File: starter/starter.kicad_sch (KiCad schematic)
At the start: 44 parts, among them J1 Conn_01x04_MountingPin, J2 Conn_01x02, J3 Conn_01x04_MountingPin, J4 Conn_01x04_MountingPin, J5 Conn_01x02_MountingPin, Q1 Q_NMOS_GDS, SW1 SW_Coded_SH-7050, SW2 SW_Coded_SH-7050, U1 MCP100-475D, U2 LM1117DT-ADJ, U3 PCF8574RGTR, U4 74HC688, U5 MCP14A1201xMNY

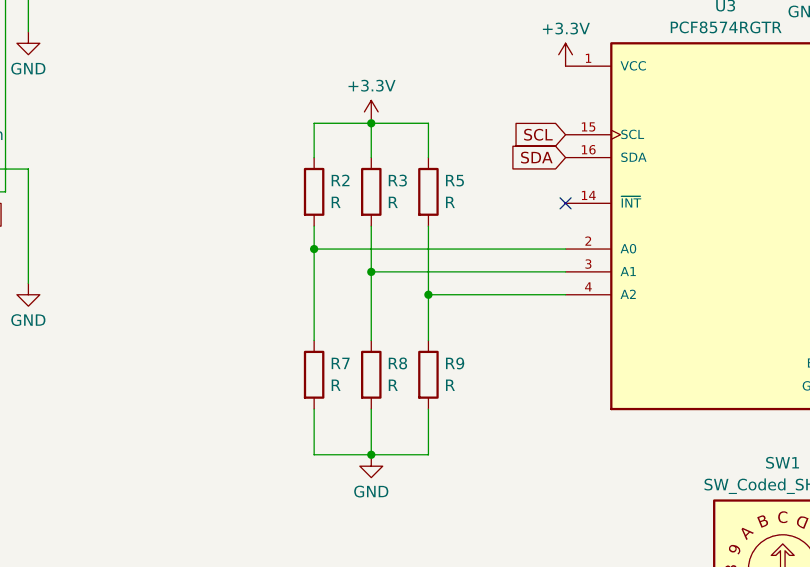
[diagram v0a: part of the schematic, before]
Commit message: updates
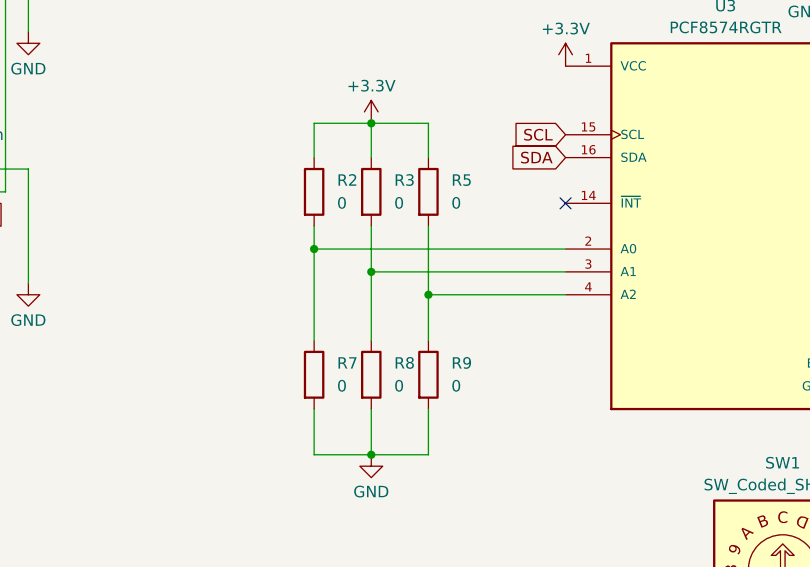
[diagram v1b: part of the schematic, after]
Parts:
- R2, R3, R5, R7, R8, R9: value R -> 0
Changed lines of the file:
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@@
 		(fields_autoplaced yes)
 		(property "Reference" "R5"
-			(at 94.488 138.4878 0)
+			(at 95.25 138.4299 0)
 			(effects
 				(font
@@
 			)
 		)
-		(property "Value" "R"
-			(at 94.488 140.9121 0)
+		(property "Value" "0"
+			(at 95.25 140.9699 0)
 			(effects
 				(font
@@
 		(fields_autoplaced yes)
 		(property "Reference" "R3"
-			(at 88.138 138.4878 0)
+			(at 88.9 138.4299 0)
 			(effects
 				(font
@@
 			)
 		)
-		(property "Value" "R"
-			(at 88.138 140.9121 0)
+		(property "Value" "0"
+			(at 88.9 140.9699 0)
 			(effects
 				(font
@@
 		(fields_autoplaced yes)
 		(property "Reference" "R9"
-			(at 94.488 158.8078 0)
+			(at 95.25 158.7499 0)
 			(effects
 				(font
@@
 			)
 		)
-		(property "Value" "R"
-			(at 94.488 161.2321 0)
+		(property "Value" "0"
+			(at 95.25 161.2899 0)
 			(effects
 				(font
@@
 		(fields_autoplaced yes)
 		(property "Reference" "R8"
-			(at 88.138 158.8078 0)
+			(at 88.9 158.7499 0)
 			(effects
 				(font
@@
 			)
 		)
-		(property "Value" "R"
-			(at 88.138 161.2321 0)
+		(property "Value" "0"
+			(at 88.9 161.2899 0)
 			(effects
 				(font
@@
 		(fields_autoplaced yes)
 		(property "Reference" "R2"
-			(at 81.788 138.4878 0)
+			(at 82.55 138.4299 0)
 			(effects
 				(font
@@
 			)
 		)
-		(property "Value" "R"
-			(at 81.788 140.9121 0)
+		(property "Value" "0"
+			(at 82.55 140.9699 0)
 			(effects
 				(font
@@
 		(fields_autoplaced yes)
 		(property "Reference" "R7"
-			(at 81.788 158.8078 0)
+			(at 82.55 158.7499 0)
 			(effects
 				(font
@@
 			)
 		)
-		(property "Value" "R"
-			(at 81.788 161.2321 0)
+		(property "Value" "0"
+			(at 82.55 161.2899 0)
 			(effects
 				(font
